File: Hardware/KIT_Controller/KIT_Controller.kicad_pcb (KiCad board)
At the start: 2 copper layers, 75 x 116.7 mm, 53 parts, among them J201 Micro_SD_Card_Det1, J202 USB_BOOT, J203 USBC, SW101 TM1000, U101 Nokia_5110_LCD, U102 CARD ?, U202 W25Q128JVS, U203 NCP1117-3.3_SOT223, U205 RP2040, U301 CC1101, Y201 Crystal

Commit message: Pivot to feather design
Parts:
- removed C101: 4.7uf, Capacitor_SMD:C_0805_2012Metric
- removed JP101: SolderJumper_2_Bridged, Jumper:SolderJumper-2_P1.3mm_Bridged_Pad1.0x1.5mm
- removed SW101: TM1000, KenwoodFox:TM1000
- removed U101: Nokia_5110_LCD, Nokia_5110-3310_LCD:Nokia_5110-3310_LCD
- added A1: Adafruit_Feather_Generic, Module:Adafruit_Feather, F.Cu at (-27.8, -102.9)
- moved C217 212.1 mm to (33.5, -91.5)
- moved D101 212.1 mm to (8.29, -4.75)
- moved D103 212.1 mm to (8.29, -42.2)
- moved D104 212.1 mm to (-4.66, -4.75)
- moved H101 212.1 mm to (28.0, -11.5)
- moved H102 212.1 mm to (-30.0, -12.0)
- moved J201 212.1 mm to (21.5, -103.4)
- moved R208 212.1 mm to (29.1, -91.5)
- moved R209 212.1 mm to (29.1, -88.6)
- moved R210 212.1 mm to (29.1, -85.6)
- moved R215 212.1 mm to (31.0, -95.6)
- moved R216 212.1 mm to (31.0, -98.5)
- moved R217 212.1 mm to (31.0, -101.5)
- moved U102 212.1 mm to (0.00, 0.00)
- moved U301 212.1 mm to (26.5, -43.1)
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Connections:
- U102 pad 11: /SCL -> unconnected-(U102-I2C_SCL-Pad11)
- U102 pad 13: /SDA -> unconnected-(U102-I2C_SDA-Pad13)

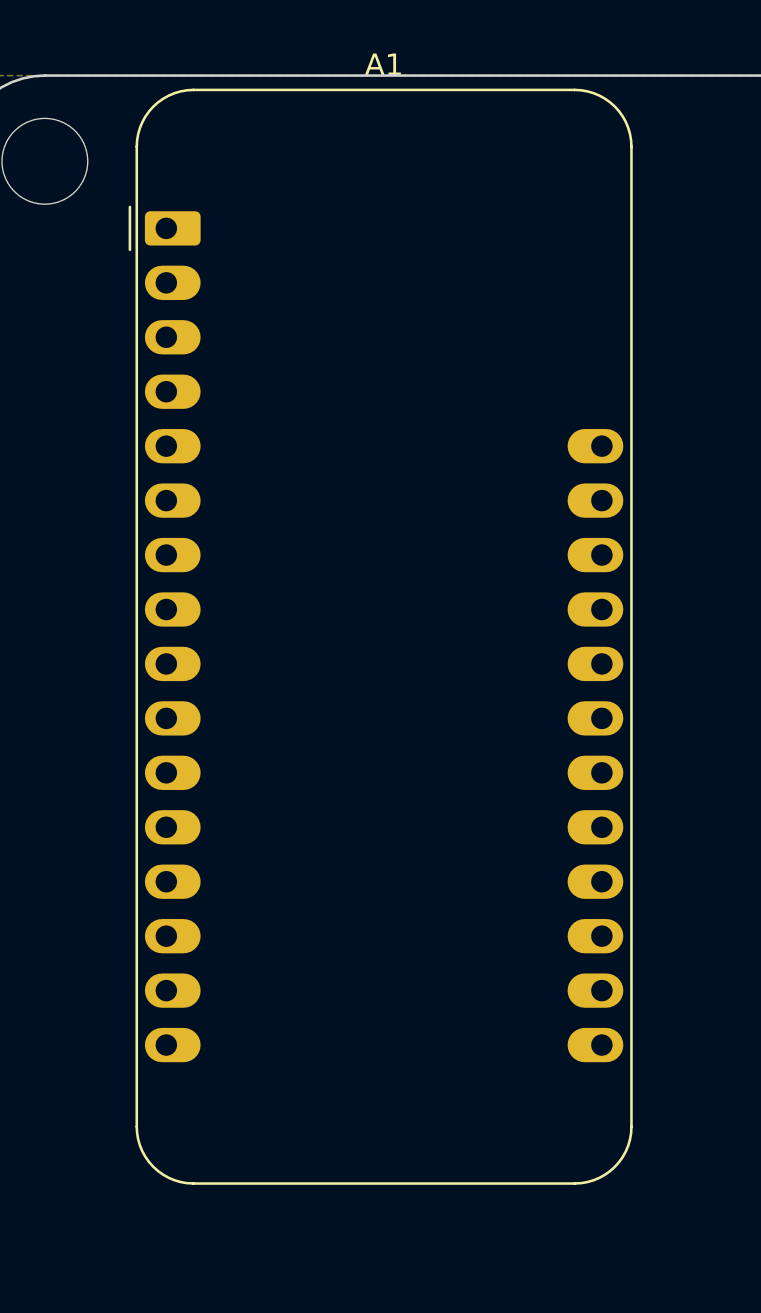
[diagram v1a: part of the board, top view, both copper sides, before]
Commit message: So near to a backplane prototype now
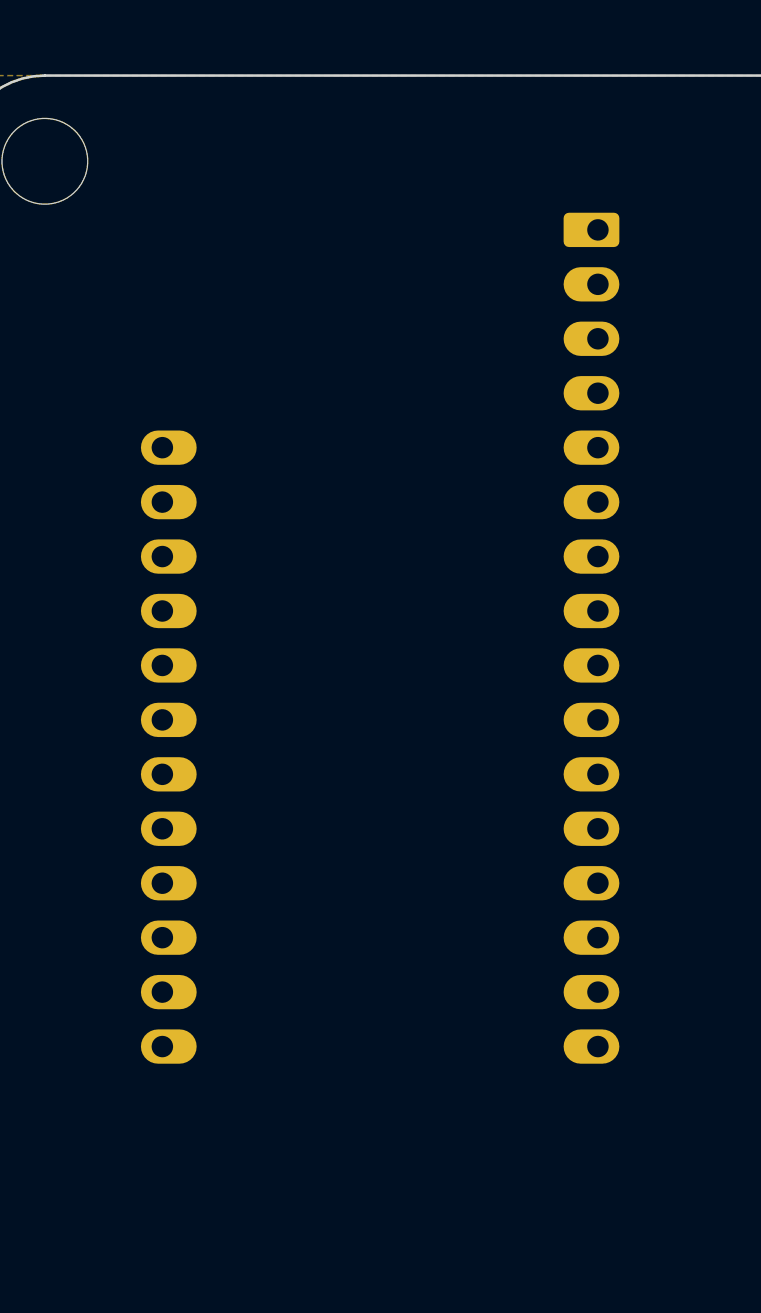
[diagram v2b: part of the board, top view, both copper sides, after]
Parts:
- A1: moved to B.Cu
- moved A1 20.1 mm to (-7.70, -102.8), turned to 180 degrees
